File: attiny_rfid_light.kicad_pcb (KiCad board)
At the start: 2 copper layers, 76 x 99.1 mm, 27 parts, among them IC1 EM4095, U1 ESP32-WROOM-32, U2 NCP1117-3.3_SOT223

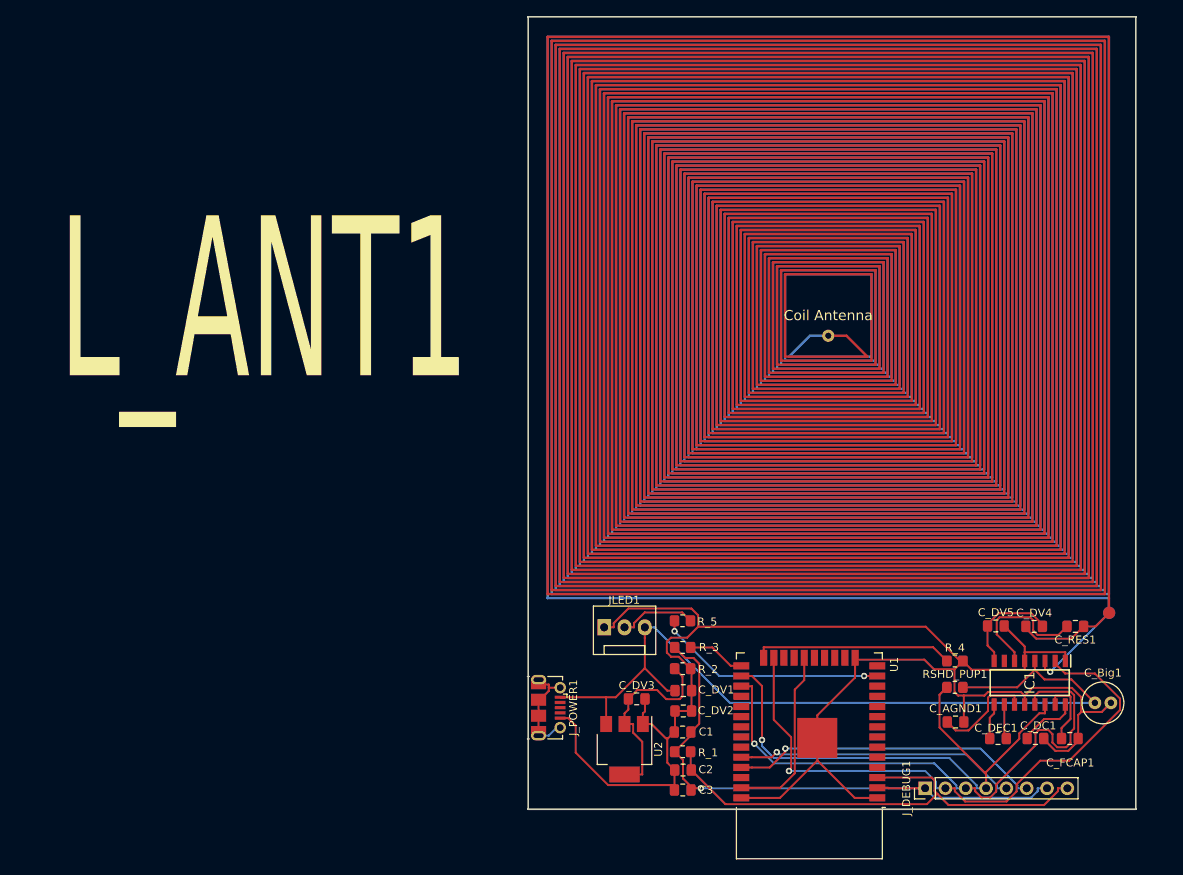
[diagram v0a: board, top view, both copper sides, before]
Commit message: v3
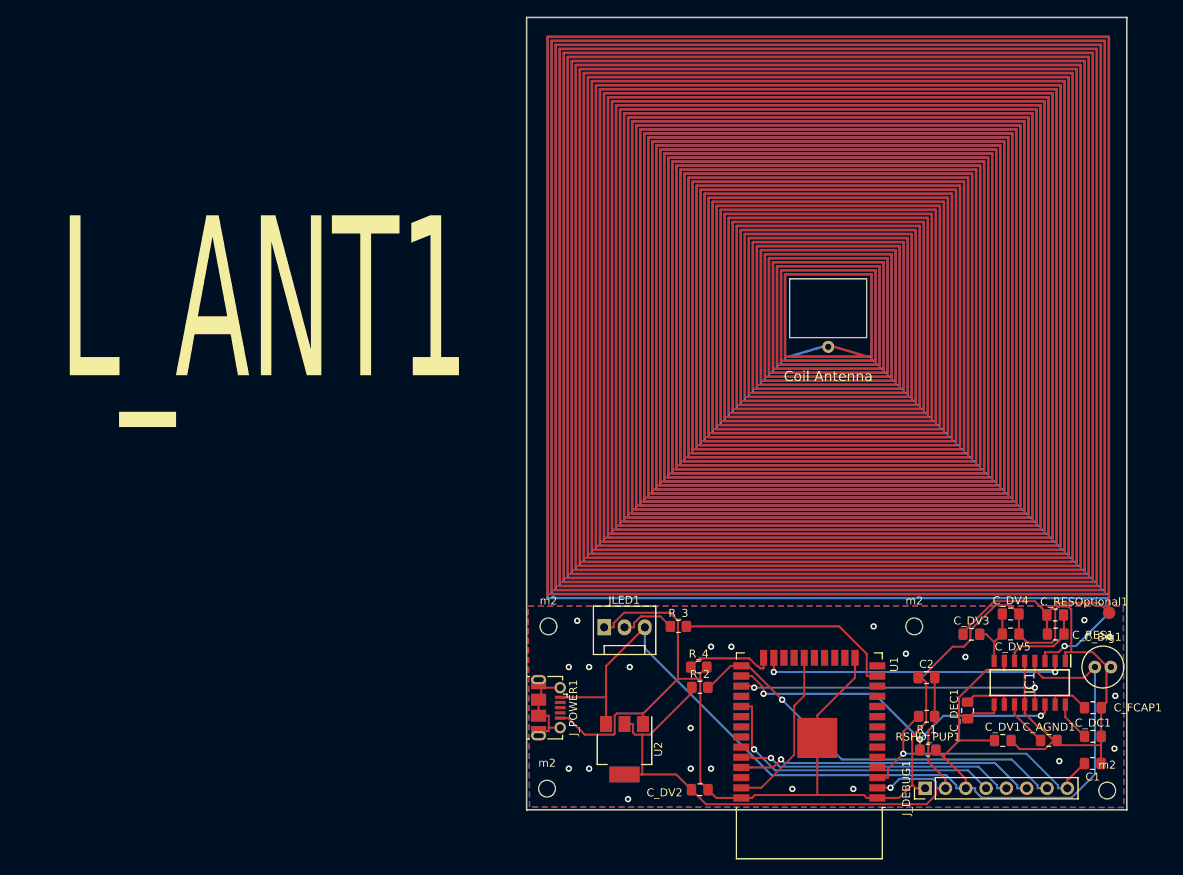
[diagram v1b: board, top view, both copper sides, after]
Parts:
- removed C3: 1uf, Capacitor_SMD:C_0805_2012Metric_Pad1.18x1.45mm_HandSolder
- removed R_5: 490, Resistor_SMD:R_0805_2012Metric_Pad1.20x1.40mm_HandSolder
- added C_RESOptional1: NA, Capacitor_SMD:C_0805_2012Metric_Pad1.18x1.45mm_HandSolder, F.Cu at (131.9, 130.6)
- added m2: MountingHole_2.1mm, MountingHole:MountingHole_2.1mm, F.Cu at (114.3, 132.1)
- added m2: MountingHole_2.1mm, MountingHole:MountingHole_2.1mm, F.Cu at (68.6, 132.1)
- added m2: MountingHole_2.1mm, MountingHole:MountingHole_2.1mm, F.Cu at (138.4, 152.6)
- added m2: MountingHole_2.1mm, MountingHole:MountingHole_2.1mm, F.Cu at (68.4, 152.4)
- C1: value 100uf -> 0.1uf
- C2: value 0.1uf -> 1uf
- C_Big1: value 10uf -> 100uf
- C_DV3: value 22uf -> 0.1nf
- C_DV4: value 0.1nf -> 3.7nf split between 2
- C_DV5: value 3.7nf -> 3.7nf split between 2
- R_2: value 3.3k -> 5k1 or 5k? was 5k og
- R_3: value 5k -> 490
- R_4: value 5k -> 5k1 og was 5k
- moved C1 51.4 mm to (136.6, 149.2), turned to 180 degrees
- moved C_DV3 42.6 mm to (121.5, 133.1)
- moved C_DV1 40.4 mm to (125.4, 146.3)
- moved C2 32.6 mm to (115.8, 138.5)
- moved R_4 32.0 mm to (87.4, 137.2)
- moved R_1 30.8 mm to (115.8, 143.3), turned to 180 degrees
- moved C_AGND1 11.9 mm to (131.1, 146.3)
- moved C_DV2 10.1 mm to (87.5, 152.5)
- moved RSHD_PUP1 8.53 mm to (116.0, 147.5)
- moved C_DC1 7.19 mm to (136.6, 145.8)
- moved C_DEC1 5.18 mm to (121.0, 142.6), turned to 90 degrees
- moved C_FCAP1 4.82 mm to (136.6, 142.2)
- moved C_Big1 4.48 mm to (136.9, 137.2)
- moved C_DV4 3.32 mm to (126.4, 130.5)
- moved R_2 3.17 mm to (87.5, 139.7)
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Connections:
- C1 pad 2: +3V3 -> Net-(C1-Pad2)
- C2 pad 2: Net-(C2-Pad2) -> +3V3
- C_DV2 pad 1: GND -> +3V3
- C_DV3 pad 2: GND -> Net-(C_DV3-Pad2)
- C_DV4 pad 1: Net-(C_DV4-Pad1) -> Net-(C_DV3-Pad2)
- C_DV4 pad 2: Net-(C_DV4-Pad2) -> GND
- C_DV5 pad 1: Net-(C_DV4-Pad2) -> Net-(C_DV3-Pad2)
- C_RES1 pad 1: Net-(C_DV4-Pad1) -> Net-(C_DV3-Pad1)
- IC1 pad 7: unconnected-(IC1-Pad7) -> +5V
- IC1 pad 8: Net-(C_DV4-Pad2) -> Net-(C_DV3-Pad2)
- J_DEBUG1 pad 1: +3V3 -> GND
- J_DEBUG1 pad 2: Net-(IC1-Pad2) -> +3V3
- J_DEBUG1 pad 3: Net-(IC1-Pad13) -> +5V
- J_DEBUG1 pad 4: Net-(IC1-Pad14) -> Net-(J_DEBUG1-Pad4)
- J_DEBUG1 pad 7: +3V3 -> Net-(J_DEBUG1-Pad7)
- J_DEBUG1 pad 8: Net-(C2-Pad2) -> Net-(C1-Pad2)
- L_ANT1 pad 1: Net-(C_DV4-Pad1) -> Net-(C_DV3-Pad1)
- R_1 pad 2: Net-(C2-Pad2) -> Net-(C1-Pad2)
- R_2 pad 1: Net-(C_DV3-Pad1) -> +3V3
- R_2 pad 2: GND -> Net-(J_DEBUG1-Pad7)
- R_3 pad 1: +3V3 -> Net-(JLED1-Pad2)
- U1 pad 13: Net-(R_5-Pad1) -> Net-(R_3-Pad2)
- U1 pad 25: Net-(R_3-Pad2) -> Net-(J_DEBUG1-Pad7)
- U1 pad 29: unconnected-(U1-Pad29) -> Net-(J_DEBUG1-Pad4)
- U1 pad 3: Net-(C2-Pad2) -> Net-(C1-Pad2)
- U2 pad 2: Net-(C_DV3-Pad1) -> +3V3
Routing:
- net Net-(C2-Pad2): track 62.4 -> 0.00 mm
- net Net-(J_DEBUG1-Pad7): track 0.00 -> 50.1 mm, vias 0 -> 1
- net Net-(J_DEBUG1-Pad4): track 0.00 -> 37.8 mm, vias 0 -> 1
- net Net-(IC1-Pad2): track 75.7 -> 38.3 mm, vias 1 -> 2
- net Net-(C1-Pad2): track 0.00 -> 37.2 mm, vias 0 -> 1
- net +5V: track 105.9 -> 138.3 mm
- net Net-(IC1-Pad13): track 70.6 -> 38.9 mm, vias 1 -> 2
- net Net-(R_5-Pad1): track 29.0 -> 0.00 mm, vias 2 -> 0
- net Net-(IC1-Pad14): track 68.5 -> 45.5 mm, vias 1 -> 3
- net Net-(R_3-Pad2): track 7.29 -> 28.1 mm
- net GND: track 215.1 -> 200.5 mm, vias 0 -> 22
- net Net-(R_4-Pad1): track 24.9 -> 11.4 mm
- net Net-(C_DV4-Pad2): track 13.2 -> 0.00 mm
- net Net-(C_DV4-Pad1): track 12.5 -> 0.00 mm
- net +3V3: track 73.5 -> 85.3 mm
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- added copper zone on B.Cu, net GND
- added copper zone on F.Cu, net GND
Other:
- board size 76 x 99.1 mm -> 75 x 99.1 mm
